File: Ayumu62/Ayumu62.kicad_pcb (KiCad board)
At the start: 2 copper layers, 337.2 x 116.5 mm, 135 parts, among them SW1 SW_Push, SW10 SW_Push, SW11 SW_Push, SW12 SW_Push, SW13 SW_Push, SW14 SW_Push, SW15 SW_Push, SW16 SW_Push, SW17 SW_Push, SW18 SW_Push, SW19 SW_Push, SW2 SW_Push, SW20 SW_Push, SW21 SW_Push, SW22 SW_Push, SW23 SW_Push, SW24 SW_Push, SW25 SW_Push, SW26 SW_Push, SW27 SW_Push, SW28 SW_Push, SW29 SW_Push, SW3 SW_Push, SW30 SW_Push, SW31 SW_Push, SW32 SW_Push, SW33 SW_Push, SW34 SW_Push, SW35 SW_Push, SW36 SW_Push, SW37 SW_Push, SW38 SW_Push, SW39 SW_Push, SW4 SW_Push, SW40 SW_Push, SW41 SW_Push, SW42 SW_Push, SW43 SW_Push, SW44 SW_Push, SW45 SW_Push, SW46 SW_Push, SW47 SW_Push, SW48 SW_Push, SW49 SW_Push, SW5 SW_Push, SW50 SW_Push, SW51 SW_Push, SW52 SW_Push, SW53 SW_Push, SW54 SW_Push, SW55 SW_Push, SW56 SW_Push, SW57 SW_Push, SW58 SW_Push, SW59 SW_Push, SW6 SW_Push, SW60 SW_Push, SW61 SW_Push, SW62 SW_Push, SW7 SW_Push, SW8 SW_Push, SW9 SW_Push, U1 YAAJ_BluePill

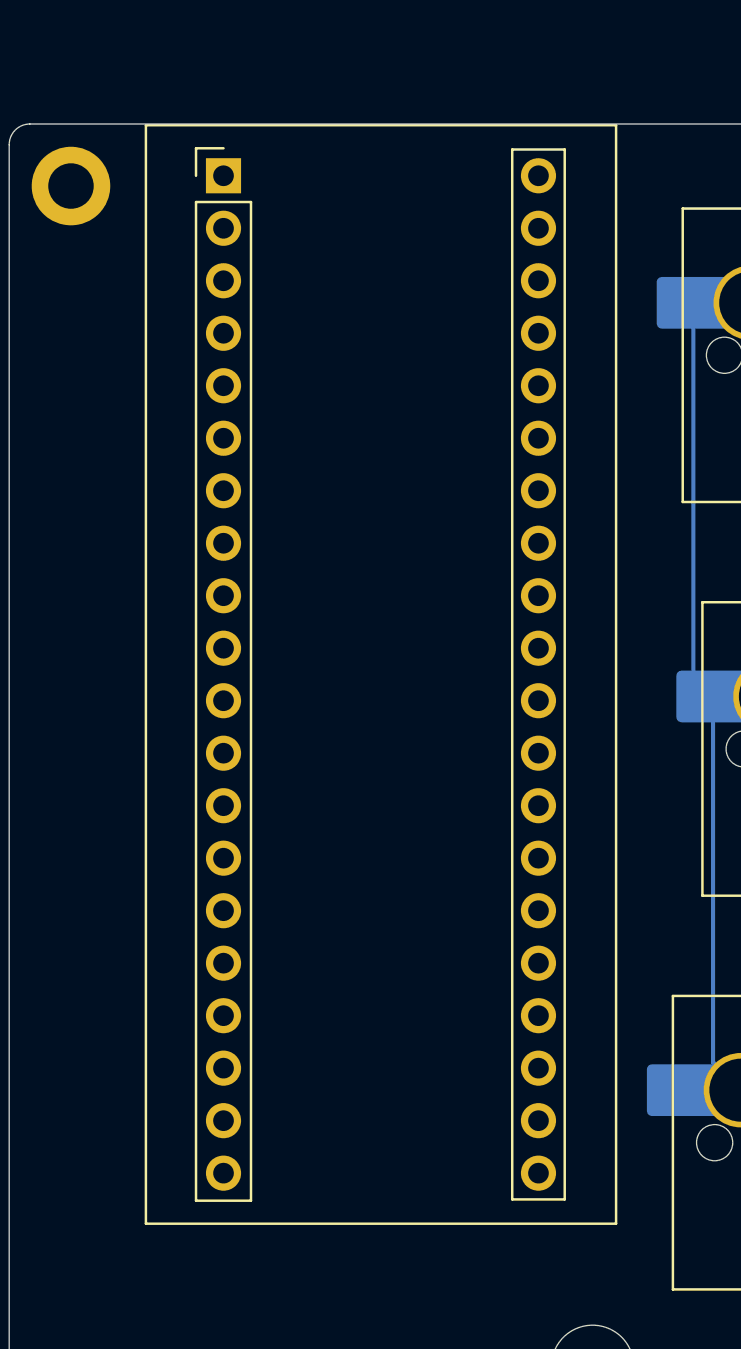
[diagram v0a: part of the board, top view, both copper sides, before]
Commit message: upd
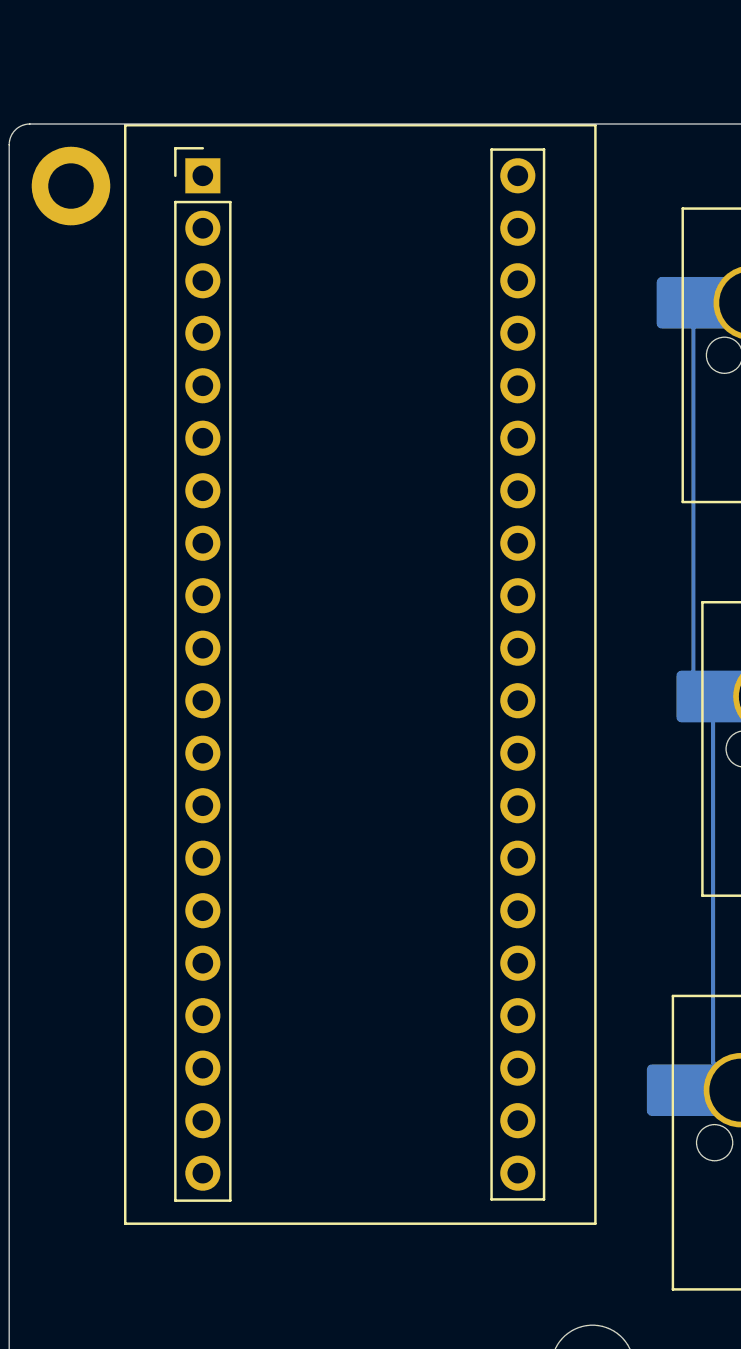
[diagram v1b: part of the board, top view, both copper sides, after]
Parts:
- moved U1 1.00 mm to (45.9, 50.4)
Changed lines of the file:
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@@
 	(footprint "YAAJ:YAAJ_BluePill_2"
 		(layer "F.Cu")
-		(at 46.88 50.37)
+		(at 45.88 50.37)
 		(descr "Through hole headers for BluePill module. No SWD breakout. Fancy silkscreen.")
 		(tags "module BlluePill Blue Pill header SWD breakout")

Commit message: upd
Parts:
- removed U1: YAAJ_BluePill, YAAJ:YAAJ_BluePill_2
- added A1: RaspberryPi_Pico, Module:RaspberryPi_Pico_Common_Unspecified, B.Cu at (72.7, 105.4)
- added REF**: Plate, Ayumu62:Plate, F.Cu at (54.2, 78.0)
- moved H10 36.1 mm to (389.3, 172.2)
- moved H9 35.4 mm to (389.3, 81.0)
- moved H7 35.3 mm to (58.2, 171.2)
- moved SW27 35.3 mm to (171.4, 95.9)
- moved D28 35.3 mm to (194.3, 103.9)
- moved D45 35.3 mm to (242.7, 103.3)
- moved D57 35.3 mm to (239.7, 162.4)
- moved SW43 35.3 mm to (203.5, 180.7)
- moved SW36 35.3 mm to (178.4, 136.4)
- moved D56 35.3 mm to (300.0, 130.1)
- moved SW28 35.3 mm to (190.0, 99.9)
- moved D55 35.3 mm to (281.4, 134.1)
- moved D37 35.3 mm to (201.3, 144.3)
- moved D52 35.3 mm to (293.2, 112.1)
- moved SW58 35.3 mm to (252.7, 156.5)
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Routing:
- net Col6: track 0.00 -> 522.2 mm, vias 0 -> 7
- net Col12: track 0.00 -> 464.0 mm, vias 0 -> 8
- net Col7: track 0.00 -> 458.2 mm, vias 0 -> 7
- net Col3: track 0.00 -> 413.9 mm, vias 0 -> 8
- net Col9: track 0.00 -> 404.4 mm, vias 0 -> 8
- net Col13: track 0.00 -> 397.7 mm, vias 0 -> 7
- net Col4: track 0.00 -> 389.2 mm, vias 0 -> 4
- net Col2: track 0.00 -> 377.5 mm, vias 0 -> 8
- net Col15: track 0.00 -> 370.0 mm, vias 0 -> 7
- net Col10: track 0.00 -> 368.3 mm, vias 0 -> 6
- net Col8: track 0.00 -> 358.9 mm, vias 0 -> 5
- net Col11: track 0.00 -> 357.2 mm, vias 0 -> 7
- net Col5: track 0.00 -> 342.3 mm, vias 0 -> 7
- net Row2: track 225.9 -> 568.2 mm, vias 0 -> 2
- net Col14: track 0.00 -> 299.4 mm, vias 0 -> 8
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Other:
- board size 337.2 x 116.5 mm -> 338.1 x 116.2 mm
